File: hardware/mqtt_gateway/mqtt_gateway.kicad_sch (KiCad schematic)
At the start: 64 parts, among them J1 awesome:RJ45-CAN, J2 Button-Sensors-MicroMatch2X03, J3 RJ45_Amphenol_RJMG1BD3B8K1ANR, J4 WAGO250-204, J5 Button-Sensors-MicroMatch2X03, U1 wuerthDebug6, U2 LD1117S33TR_SOT223, U3 PESD2CAN, U4 MCP2562-E-SN, U6 ESP32-WROOM-32, U7 LAN8720A

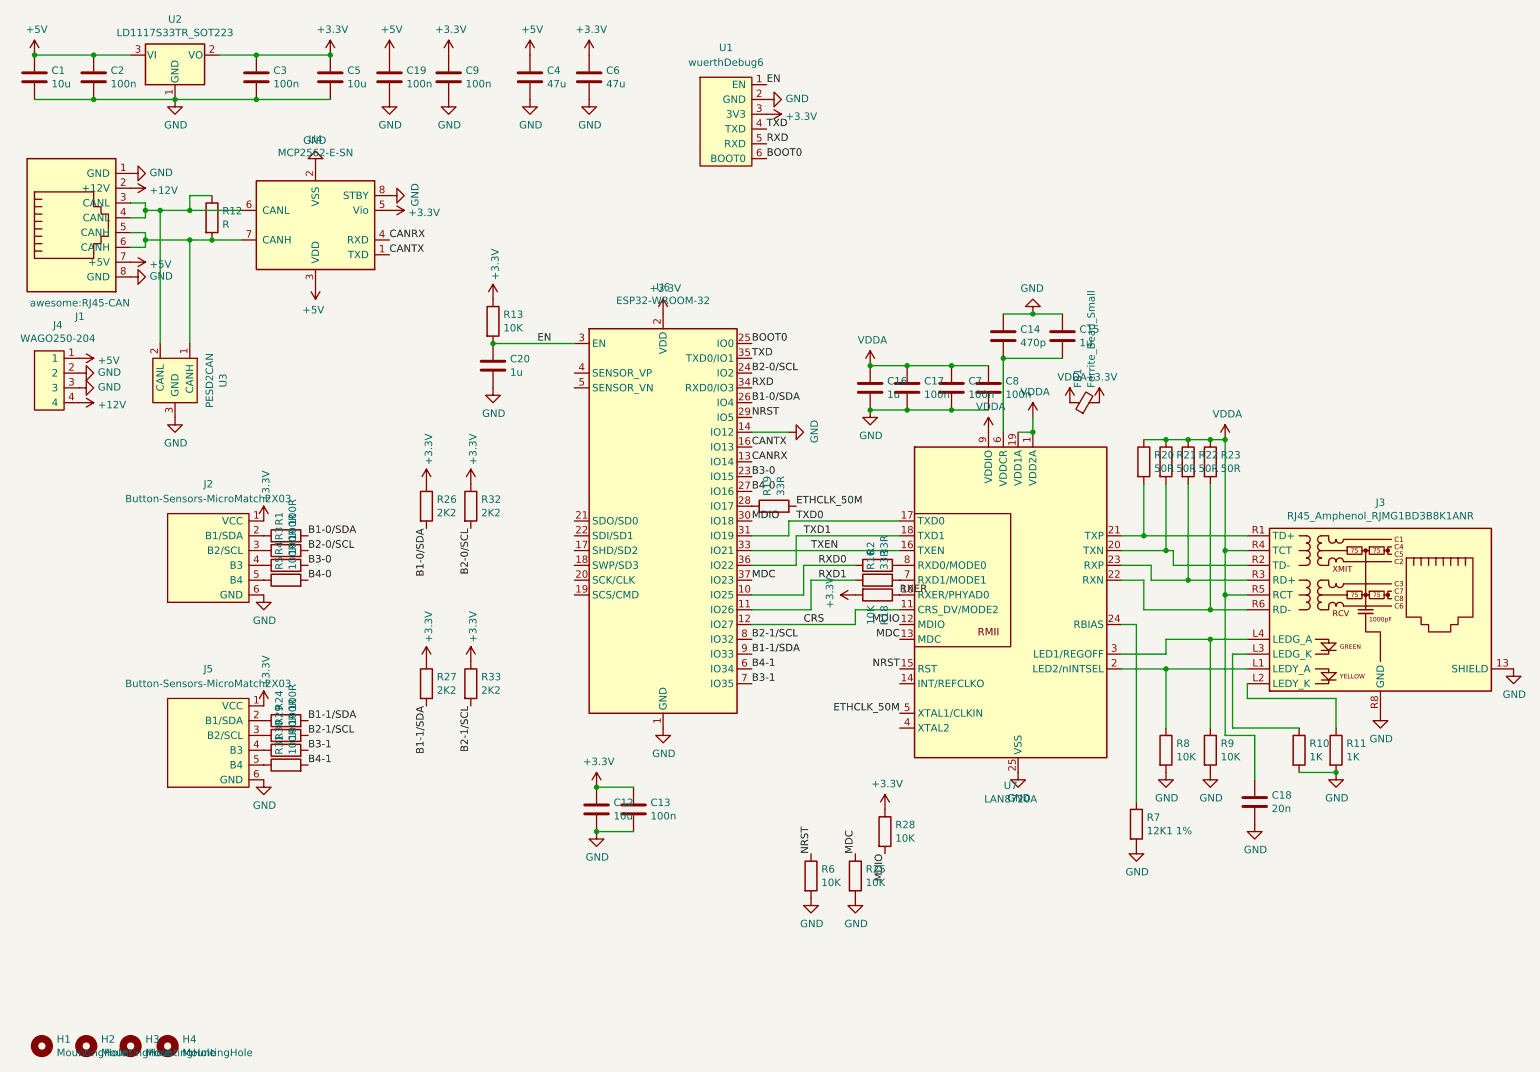
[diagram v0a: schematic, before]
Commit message: feat: Prepare mqtt gateway 3.0
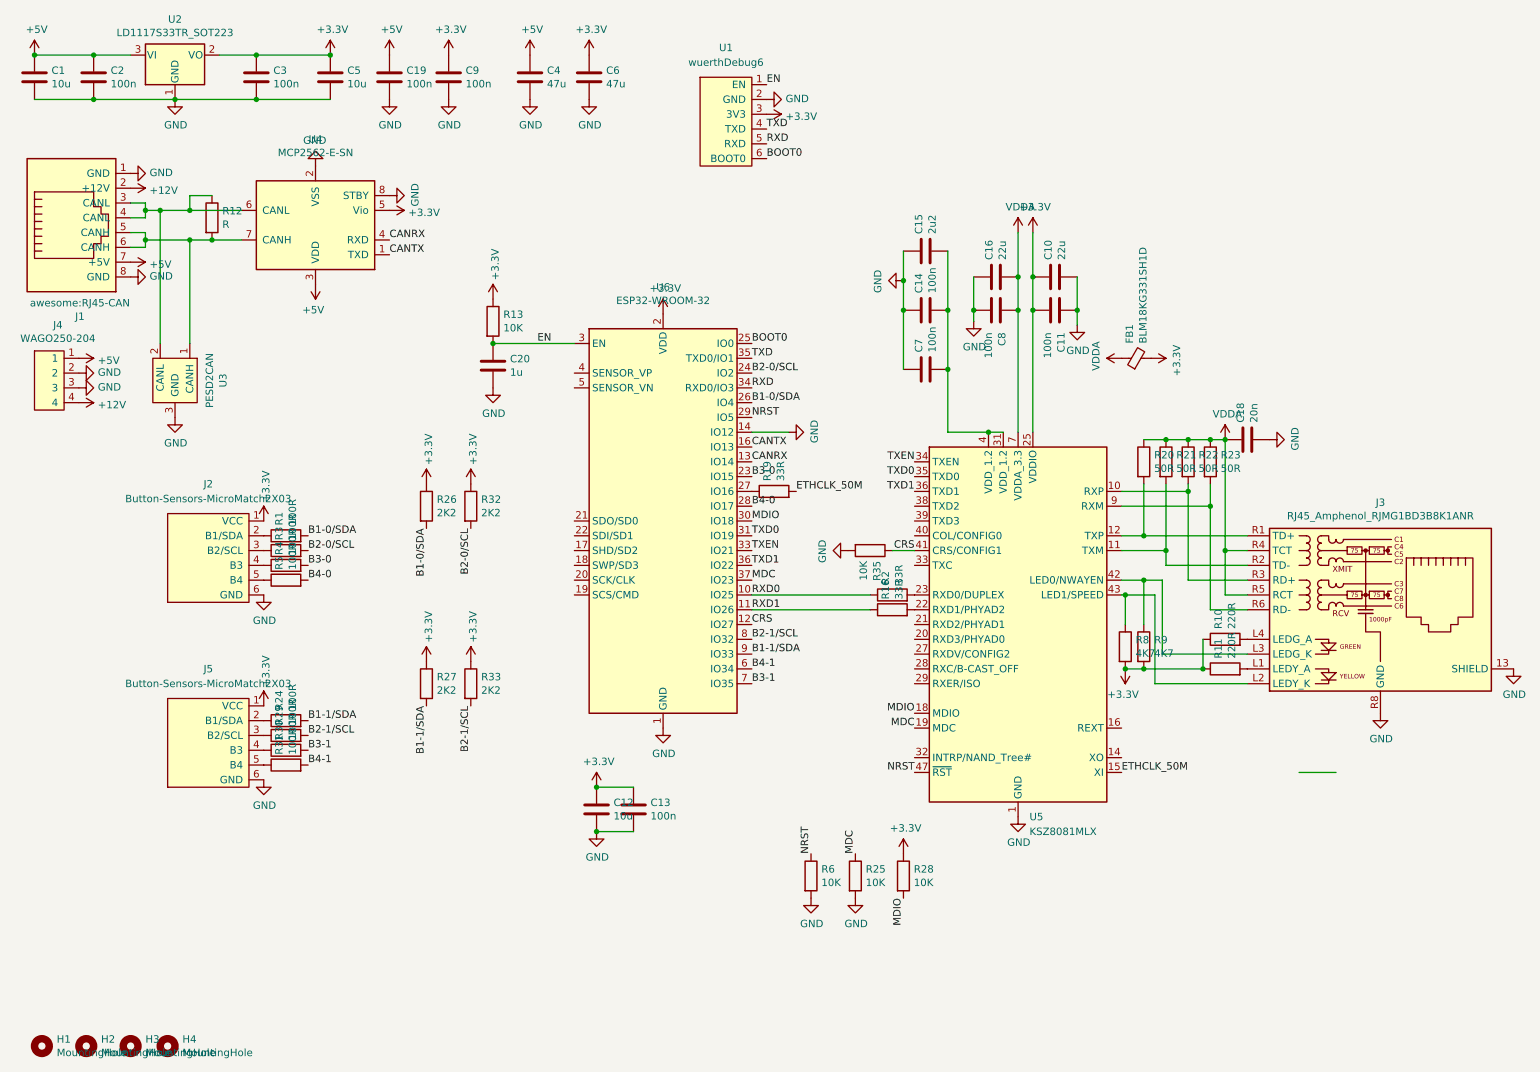
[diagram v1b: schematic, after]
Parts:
- removed C17: 100n, Capacitor_SMD:C_0402_1005Metric_Pad0.74x0.62mm_HandSolder, symbol Device:C
- removed R18: 10K, Resistor_SMD:R_0402_1005Metric_Pad0.72x0.64mm_HandSolder, symbol Device:R
- removed R7: 12K1 1%, Resistor_SMD:R_0603_1608Metric_Pad0.98x0.95mm_HandSolder, symbol Device:R
- removed U7: LAN8720A, Package_DFN_QFN:QFN-24-1EP_4x4mm_P0.5mm_EP2.6x2.6mm, symbol Interface_Ethernet:LAN8720A
- added C10: 22u, Capacitor_SMD:C_0805_2012Metric_Pad1.18x1.45mm_HandSolder, symbol Device:C
- added C11: 100n, Capacitor_SMD:C_0603_1608Metric_Pad1.08x0.95mm_HandSolder, symbol Device:C
- added R35: 10K, Resistor_SMD:R_0603_1608Metric_Pad0.98x0.95mm_HandSolder, symbol Device:R
- added U5: KSZ8081MLX, Package_QFP:LQFP-48_7x7mm_P0.5mm, symbol Interface_Ethernet:KSZ8081MLX
- C14: value 470p -> 100n; footprint Capacitor_SMD:C_0402_1005Metric_Pad0.74x0.62mm_HandSolder -> Capacitor_SMD:C_0603_1608Metric_Pad1.08x0.95mm_HandSolder
- C15: value 1u -> 2u2; footprint Capacitor_SMD:C_0402_1005Metric_Pad0.74x0.62mm_HandSolder -> Capacitor_SMD:C_0603_1608Metric_Pad1.08x0.95mm_HandSolder
- C16: value 1u -> 22u; footprint Capacitor_SMD:C_0402_1005Metric_Pad0.74x0.62mm_HandSolder -> Capacitor_SMD:C_0805_2012Metric_Pad1.18x1.45mm_HandSolder
- C7, C8: footprint Capacitor_SMD:C_0402_1005Metric_Pad0.74x0.62mm_HandSolder -> Capacitor_SMD:C_0603_1608Metric_Pad1.08x0.95mm_HandSolder
- FB1: value Ferrite_Bead_Small -> BLM18KG331SH1D
- R10, R11: value 1K -> 220R
- R16, R2: footprint Resistor_SMD:R_0402_1005Metric_Pad0.72x0.64mm_HandSolder -> Resistor_SMD:R_0603_1608Metric_Pad0.98x0.95mm_HandSolder
- R8, R9: value 10K -> 4K7
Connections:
- net +3.3V: now also R10.1, R11.1, R8.2, R9.2, C10.1, C11.2, U5.25 (VDDIO)
- net B4-0: now also U6.28 (IO17); no longer U6.27 (IO16)
- net CRS: now also R35.1, U5.41 (CRS/CONFIG1)
- net ETHCLK_50M: now also U5.15 (XI)
- net GND: now also C16.1, C7.1, C10.2, C11.1, R35.2, U5.1 (GND), U5.13 (GND), U5.17 (GND), U5.2 (GND), U5.24 (GND), U5.3 (GND), U5.30 (GND), U5.37 (GND); no longer C16.2, C7.2, R10.2, R11.2, R8.2, R9.2
- net MDC: now also U5.19 (MDC)
- net MDIO: now also U5.18 (MDIO)
- net NRST: now also U5.47 (~{RST})
- net TXD0: now also U5.35 (TXD0)
- net TXD1: now also U5.36 (TXD1)
- net TXEN: now also U5.34 (TXEN)
- net VDDA: now also C16.2, U5.7 (VDDA_3.3); no longer C16.1, C7.1
- net at R19.1: now also U6.27 (IO16); no longer U6.28 (IO17)
- net at J3.L1 (LEDY_A): now also R11.2; no longer R8.1
- net at J3.L2 (LEDY_K): now also R8.1, U5.43 (LED1/SPEED); no longer R11.1
- net at J3.L3 (LEDG_K): now also R9.1, U5.42 (LED0/NWAYEN); no longer R10.1
- net at J3.L4 (LEDG_A): now also R10.2; no longer R9.1
- net at J3.R1 (TD+), R20.2: now also U5.12 (TXP)
- net at J3.R2 (TD-), R21.2: now also U5.11 (TXM)
- net at J3.R3 (RD+), R22.2: now also U5.10 (RXP)
- net at J3.R6 (RD-), R23.2: now also U5.9 (RXM)
- net at C14.2, C15.2: now also C7.2, U5.31 (VDD_1.2), U5.4 (VDD_1.2)
- net at R16.2: now also U5.22 (RXD1/PHYAD2)
- net at R2.2: now also U5.23 (RXD0/DUPLEX)
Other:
- moved on the sheet: C14, C15, C16, C18, C7, C8, FB1, R10, R11, R16, R19, R2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
